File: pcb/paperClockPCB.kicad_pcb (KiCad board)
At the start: 2 copper layers, 13 parts, among them J1 USB_B_Micro, J2 Conn_01x02_Female, J3 Conn_01x08, J4 Conn_01x02, J5 Conn_01x02, J6 AVR-ISP-6, M1 DS1337, U1 ATmega328P-PU, Y1 Crystal

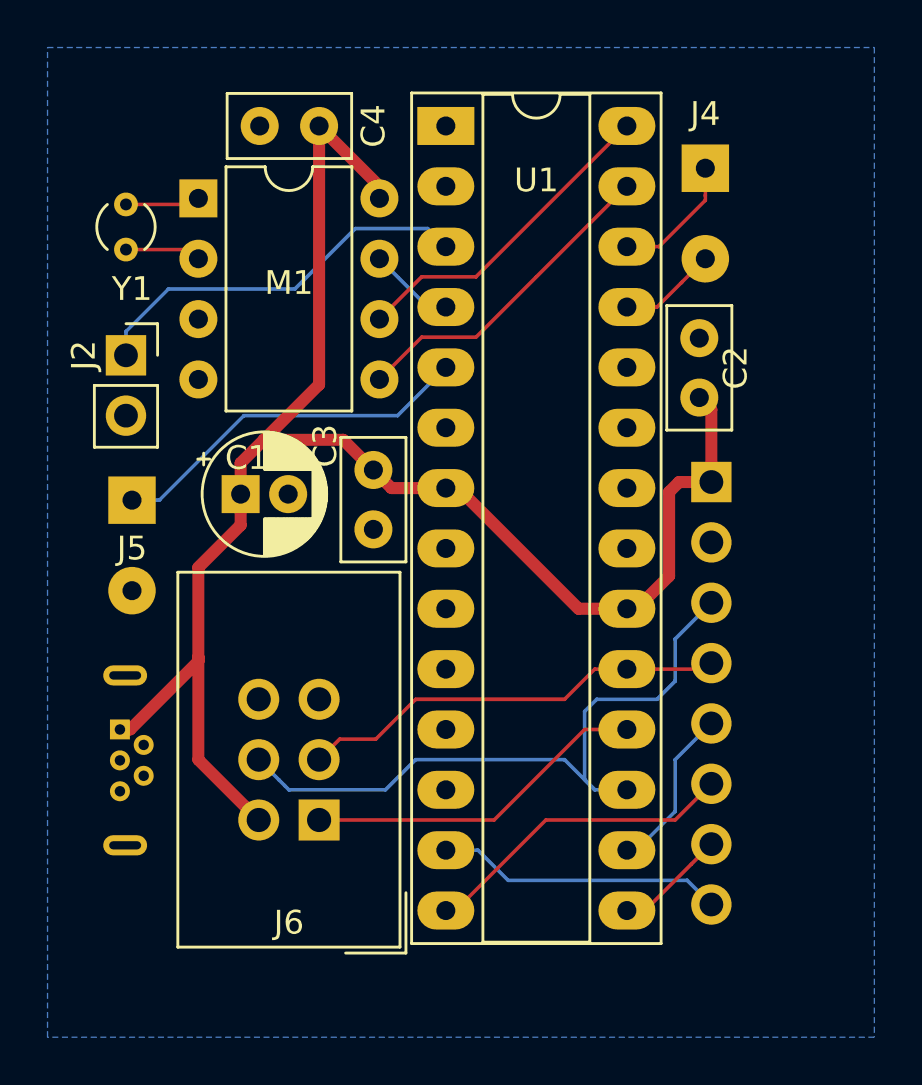
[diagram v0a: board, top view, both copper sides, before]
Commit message: PCB v0.1
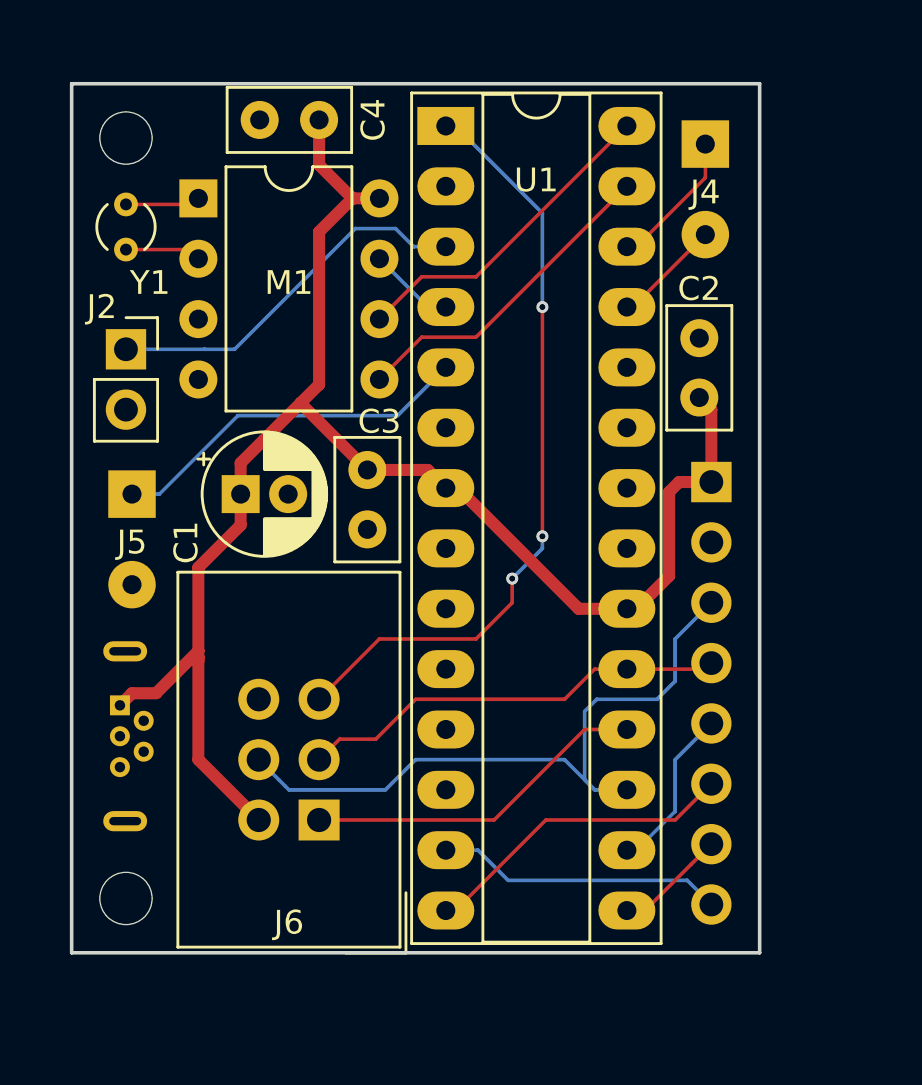
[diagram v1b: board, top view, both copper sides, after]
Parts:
- added REF**: MountingHole_2.2mm_M2_ISO7380, MountingHole:MountingHole_2.2mm_M2_ISO7380, F.Cu at (136.4, 84.3)
- added REF**: MountingHole_2.2mm_M2_ISO7380, MountingHole:MountingHole_2.2mm_M2_ISO7380, F.Cu at (136.4, 52.3)
- moved J4 1.02 mm to (160.8, 52.6)
- moved J1 1.02 mm to (136.1, 76.2)
- moved C3 0.25 mm to (146.6, 68.8)
- moved C4 0.25 mm to (144.5, 51.6)
- moved J2 0.25 mm to (136.4, 61.2)
- moved J5 0.25 mm to (136.7, 67.3)
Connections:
- J1 pad 6: Net-(J1-Pad6) -> GND
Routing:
- net Net-(J6-Pad5): track 0.00 -> 32.3 mm, vias 0 -> 3
- net VCC: track 72.1 -> 69.9 mm
- net /TX: track 16.6 -> 15.9 mm
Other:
- board outline added: 29 x 36.6 mm
